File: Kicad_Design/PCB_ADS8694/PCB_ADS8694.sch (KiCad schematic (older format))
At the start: 46 parts, among them J1 Screw_Terminal_01x03_Alimenta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, J4 Conn_02x06_Male_Pmod_Spartan6, J5 Screw_Terminal_01x02_CH3, J6 Screw_Terminal_01x02_CH2, J7 Screw_Terminal_01x02_CH1, J8 Screw_Terminal_01x02_CH0, U1 LM7805_TO220, U2 AD8221, U3 AD8221, U4 ADS8694, U5 AD8221, U6 AD8221

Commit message: PCB V1
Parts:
- removed U4: ADS8694, Package_SO:TSSOP-38_4.4x9.7mm_P0.5mm, symbol PCB_ADS8694-rescue:ADS8694-Analog_ADC-PCB_ADS8694-rescue
- added U4: ADS8694_Vers2, Package_SO:TSSOP-38_4.4x9.7mm_P0.5mm, symbol ads8694_vers2:ADS8694_Vers2
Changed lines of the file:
@@
 EESchema Schematic File Version 4
-LIBS:PCB_ADS8694-cache
 EELAYER 29 0
 EELAYER END
@@
 F 3 "~" H 4950 1850 50  0001 C CNN
 	1    4950 1850
-	1    0    0    -1
-$EndComp
-$Comp
-L PCB_ADS8694-rescue:ADS8694-Analog_ADC-PCB_ADS8694-rescue U4
-U 1 1 5CCB2EF2
-P 5750 4500
-F 0 "U4" H 5750 4550 50  0000 C CNN
-F 1 "ADS8694" H 5750 4450 50  0000 C CNN
-F 2 "Package_SO:TSSOP-38_4.4x9.7mm_P0.5mm" H 5750 4500 50  0001 C CNN
-F 3 "http://www.ti.com/lit/ds/symlink/ads8694.pdf" H 6700 5800 50  0001 C CNN
-	1    5750 4500
 	1    0    0    -1
 $EndComp
@@
 L power:GNDD #PWR0119
 U 1 1 5CD863F9
-P 6100 5800
-F 0 "#PWR0119" H 6100 5550 50  0001 C CNN
-F 1 "GNDD" H 6104 5645 50  0000 C CNN
-F 2 "" H 6100 5800 50  0001 C CNN
-F 3 "" H 6100 5800 50  0001 C CNN
-	1    6100 5800
+P 6050 5800
+F 0 "#PWR0119" H 6050 5550 50  0001 C CNN
+F 1 "GNDD" H 6054 5645 50  0000 C CNN
+F 2 "" H 6050 5800 50  0001 C CNN
+F 3 "" H 6050 5800 50  0001 C CNN
+	1    6050 5800
 	1    0    0    -1
 $EndComp
@@
 Text GLabel 5750 3100 1    50   Input ~ 0
 AVDD
-Wire Wire Line
-	5650 5800 5650 5875
-Wire Wire Line
-	5450 5875 5450 5800
-Wire Wire Line
-	5550 5800 5550 5875
-Connection ~ 5550 5875
-Wire Wire Line
-	5550 5875 5450 5875
 $Comp
 L power:GNDA #PWR034
 U 1 1 5CEF30B1
-P 5650 5875
-F 0 "#PWR034" H 5650 5625 50  0001 C CNN
-F 1 "GNDA" H 5655 5702 50  0000 C CNN
-F 2 "" H 5650 5875 50  0001 C CNN
-F 3 "" H 5650 5875 50  0001 C CNN
-	1    5650 5875
-	1    0    0    -1
-$EndComp
-Wire Wire Line
-	5750 5800 5750 5875
-Wire Wire Line
-	5750 5875 5650 5875
-Connection ~ 5650 5875
-Wire Wire Line
-	5850 5800 5850 5875
-Wire Wire Line
-	5850 5875 5750 5875
-Connection ~ 5750 5875
-Wire Wire Line
-	5550 5875 5650 5875
+P 5600 5900
+F 0 "#PWR034" H 5600 5650 50  0001 C CNN
+F 1 "GNDA" H 5605 5727 50  0000 C CNN
+F 2 "" H 5600 5900 50  0001 C CNN
+F 3 "" H 5600 5900 50  0001 C CNN
+	1    5600 5900
+	1    0    0    -1
+$EndComp
 $Comp
 L Device:C C7
@@
 Text GLabel 4750 1750 0    50   Input ~ 0
 CS
+$Comp
+L ads8694_vers2:ADS8694_Vers2 U4
+U 1 1 5CE32CBF
+P 5750 4500
+F 0 "U4" H 5750 5981 50  0000 C CNN
+F 1 "ADS8694_Vers2" H 5750 5890 50  0000 C CNN
+F 2 "Package_SO:TSSOP-38_4.4x9.7mm_P0.5mm" H 5750 4500 50  0001 C CNN
+F 3 "http://www.ti.com/lit/ds/symlink/ads8694.pdf" H 6700 5800 50  0001 C CNN
+	1    5750 4500
+	1    0    0    -1
+$EndComp
+Wire Wire Line
+	5400 5800 5400 5900
+Wire Wire Line
+	5400 5900 5500 5900
+Wire Wire Line
+	5500 5800 5500 5900
+Connection ~ 5500 5900
+Wire Wire Line
+	5500 5900 5600 5900
+Wire Wire Line
+	5600 5800 5600 5900
+Connection ~ 5600 5900
+Wire Wire Line
+	5700 5800 5700 5900
+Wire Wire Line
+	5700 5900 5625 5900
+Wire Wire Line
+	5800 5800 5800 5900
+Wire Wire Line
+	5800 5900 5700 5900
+Connection ~ 5700 5900
 $EndSCHEMATC

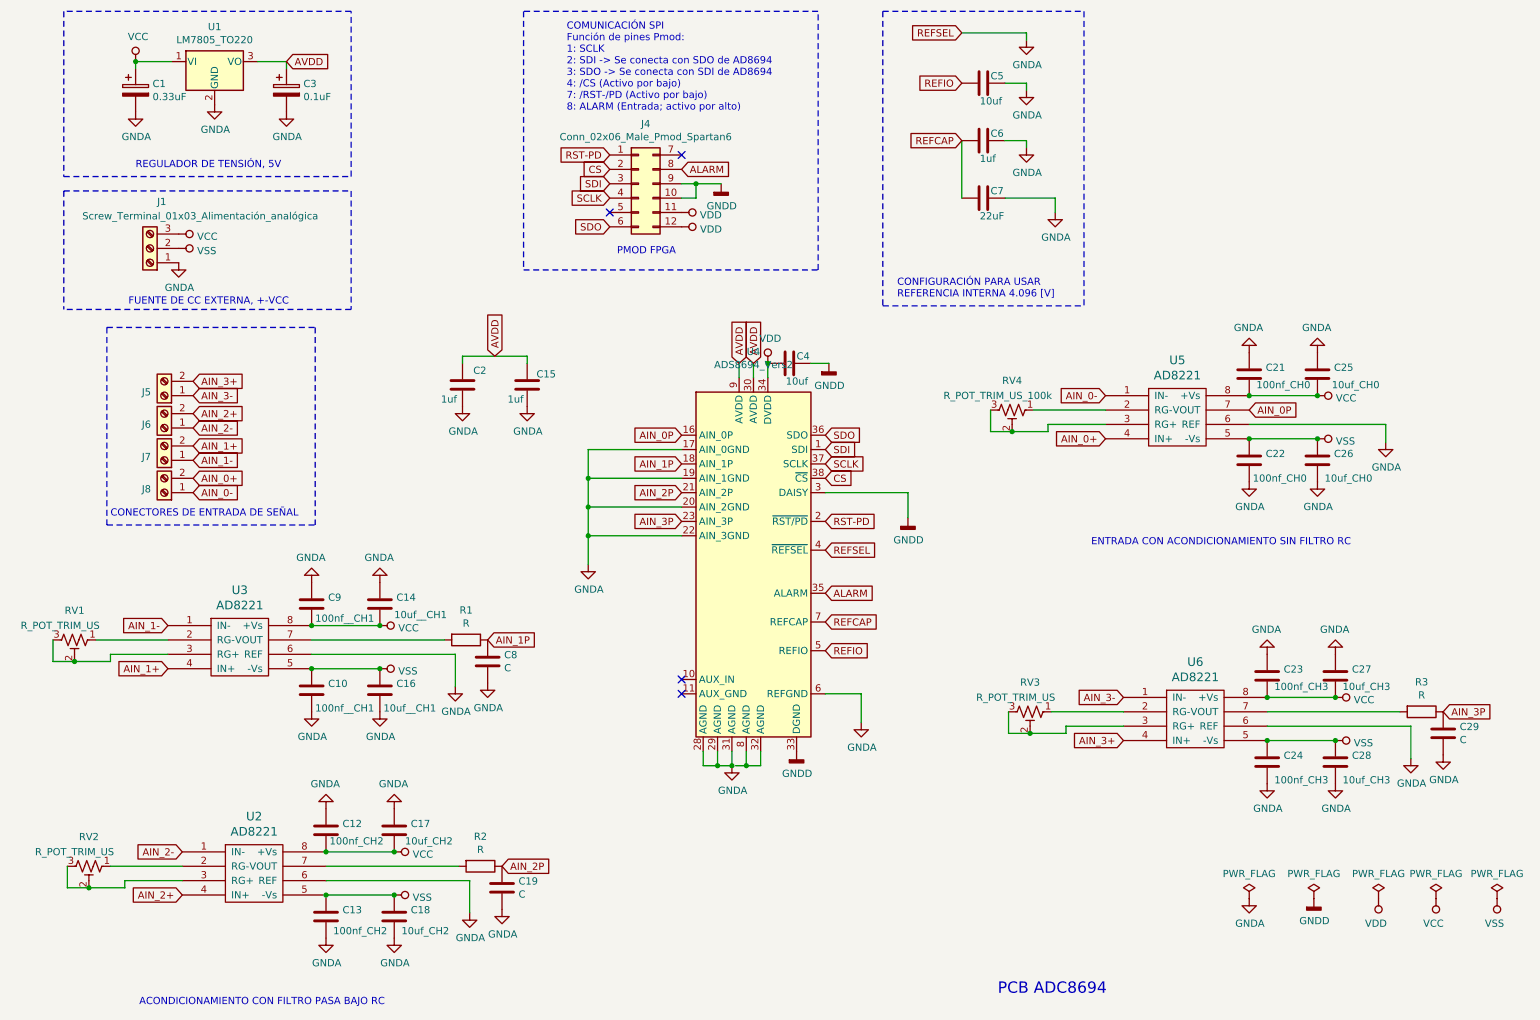
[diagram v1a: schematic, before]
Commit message: PCB V1
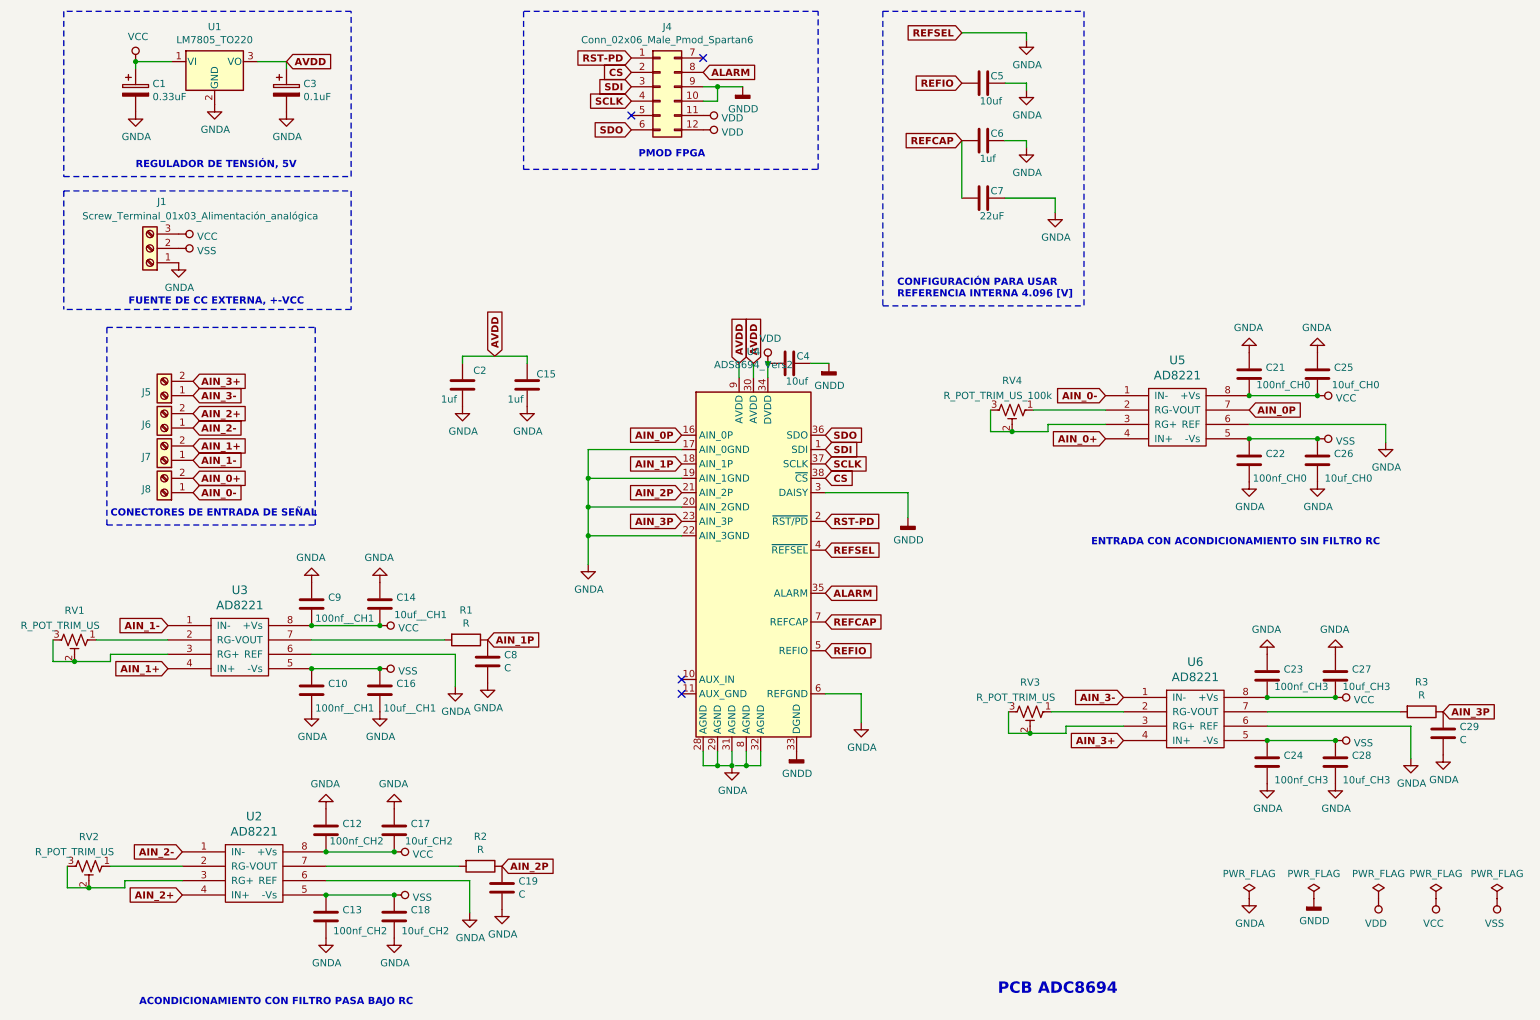
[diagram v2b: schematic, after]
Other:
- note removed: "COMUNICACIÓN SPI\nFunción de pines Pmod:\n1: SCLK\n2: SDI -> Se conecta con SDO de AD8694\n3: SDO -> Se conecta con SDI de AD8694\n4: /CS (Activo por bajo)\n7: /RST-/PD (Activo por bajo)\n8: ALARM (Entrada; activo por alto)"
- moved on the sheet: J4
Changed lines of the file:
@@
 L Connector_Generic:Conn_02x06_Top_Bottom J4
 U 1 1 5CCB59D8
-P 4950 1850
-F 0 "J4" H 5000 2267 50  0000 C CNN
-F 1 "Conn_02x06_Male_Pmod_Spartan6" H 5000 2176 50  0000 C CNN
-F 2 "Connector_PinHeader_2.54mm:PinHeader_2x06_P2.54mm_Horizontal" H 4950 1850 50  0001 C CNN
-F 3 "~" H 4950 1850 50  0001 C CNN
-	1    4950 1850
+P 5100 1175
+F 0 "J4" H 5150 1592 50  0000 C CNN
+F 1 "Conn_02x06_Male_Pmod_Spartan6" H 5150 1501 50  0000 C CNN
+F 2 "Connector_PinHeader_2.54mm:PinHeader_2x06_P2.54mm_Horizontal" H 5100 1175 50  0001 C CNN
+F 3 "~" H 5100 1175 50  0001 C CNN
+	1    5100 1175
 	1    0    0    -1
 $EndComp
@@
 Wire Wire Line
 	2500 1000 2500 1050
-Text GLabel 6250 4400 2    50   Input ~ 0
+Text GLabel 6250 4400 2    50   Input ~ 6
 REFSEL
-Text GLabel 6250 4700 2    50   Input ~ 0
+Text GLabel 6250 4700 2    50   Input ~ 6
 ALARM
-Text GLabel 6250 4900 2    50   Input ~ 0
+Text GLabel 6250 4900 2    50   Input ~ 6
 REFCAP
-Text GLabel 6250 5100 2    50   Input ~ 0
+Text GLabel 6250 5100 2    50   Input ~ 6
 REFIO
-Text GLabel 6250 4200 2    50   Input ~ 0
+Text GLabel 6250 4200 2    50   Input ~ 6
 RST-PD
-Text GLabel 6250 3900 2    50   Input ~ 0
+Text GLabel 6250 3900 2    50   Input ~ 6
 CS
-Text GLabel 6250 3800 2    50   Input ~ 0
+Text GLabel 6250 3800 2    50   Input ~ 6
 SCLK
-Text GLabel 6250 3700 2    50   Input ~ 0
+Text GLabel 6250 3700 2    50   Input ~ 6
 SDI
-Text GLabel 6250 3600 2    50   Input ~ 0
+Text GLabel 6250 3600 2    50   Input ~ 6
 SDO
-Text GLabel 5250 3800 0    50   Input ~ 0
+Text GLabel 5250 3800 0    50   Input ~ 6
 AIN_1P
-Text GLabel 5250 4000 0    50   Input ~ 0
+Text GLabel 5250 4000 0    50   Input ~ 6
 AIN_2P
-Text GLabel 5250 4200 0    50   Input ~ 0
+Text GLabel 5250 4200 0    50   Input ~ 6
 AIN_3P
-Text GLabel 7200 800  0    50   Input ~ 0
+Text GLabel 7200 800  0    50   Input ~ 6
 REFSEL
-Text GLabel 7200 1150 0    50   Input ~ 0
+Text GLabel 7200 1150 0    50   Input ~ 6
 REFIO
-Text GLabel 7200 1550 0    50   Input ~ 0
+Text GLabel 7200 1550 0    50   Input ~ 6
 REFCAP
 Wire Wire Line
 	7200 1550 7200 1950
-Text Notes 6750 2650 0    50   ~ 0
+Text Notes 6750 2650 0    50   ~ 6
 CONFIGURACIÓN PARA USAR\nREFERENCIA INTERNA 4.096 [V]\n
-Text Notes 4800 2350 0    50   ~ 0
+Text Notes 4950 1675 0    50   ~ 6
 PMOD FPGA
 Wire Notes Line
@@
 Wire Notes Line
 	2950 650  950  650
-Text Notes 1450 1750 0    50   ~ 0
+Text Notes 1450 1750 0    50   ~ 6
 REGULADOR DE TENSIÓN, 5V\n
-Text Notes 7450 7500 0    79   ~ 0
+Text Notes 7450 7500 0    79   ~ 6
 PCB ADC8694
 Wire Notes Line
 	950  650  950  1800
-Text GLabel 4750 1950 0    50   Input ~ 0
+Text GLabel 4900 1275 0    50   Input ~ 6
 SCLK
-Text GLabel 4750 2150 0    50   Input ~ 0
+Text GLabel 4900 1475 0    50   Input ~ 6
 SDO
-Text GLabel 4750 1850 0    50   Input ~ 0
+Text GLabel 4900 1175 0    50   Input ~ 6
 SDI
-Text Notes 4450 1350 0    50   ~ 0
-COMUNICACIÓN SPI\nFunción de pines Pmod:\n1: SCLK\n2: SDI -> Se conecta con SDO de AD8694\n3: SDO -> Se conecta con SDI de AD8694\n4: /CS (Activo por bajo)\n7: /RST-/PD (Activo por bajo)\n8: ALARM (Entrada; activo por alto)
-Wire Notes Line
-	4150 2450 6200 2450
-Wire Notes Line
-	6200 2450 6200 650
 Wire Notes Line
 	6200 650  4150 650
-Text Notes 1400 2700 0    50   ~ 0
+Text Notes 1400 2700 0    50   ~ 6
 FUENTE DE CC EXTERNA, +-VCC
 Wire Notes Line
@@
 Wire Wire Line
 	5250 3700 4600 3700
-NoConn ~ 4750 2050
-NoConn ~ 5250 1650
+NoConn ~ 4900 1375
+NoConn ~ 5400 975
 $Comp
 L power:GNDD #PWR0118
 U 1 1 5CD843B0
-P 5525 1850
-F 0 "#PWR0118" H 5525 1600 50  0001 C CNN
-F 1 "GNDD" H 5529 1695 50  0000 C CNN
-F 2 "" H 5525 1850 50  0001 C CNN
-F 3 "" H 5525 1850 50  0001 C CNN
-	1    5525 1850
+P 5675 1175
+F 0 "#PWR0118" H 5675 925 50  0001 C CNN
+F 1 "GNDD" H 5679 1020 50  0000 C CNN
+F 2 "" H 5675 1175 50  0001 C CNN
+F 3 "" H 5675 1175 50  0001 C CNN
+	1    5675 1175
 	1    0    0    -1
 $EndComp
@@
 	1    0    0    -1
 $EndComp
-Text GLabel 9200 3425 2    50   Input ~ 0
+Text GLabel 9200 3425 2    50   Input ~ 6
 AIN_0P
-Text GLabel 8200 3625 0    50   Input ~ 0
+Text GLabel 8200 3625 0    50   Input ~ 6
 AIN_0+
-Text GLabel 8200 3325 0    50   Input ~ 0
+Text GLabel 8200 3325 0    50   Input ~ 6
 AIN_0-
 $Comp
@@
 	0    1    1    0
 $EndComp
-Text GLabel 8325 5425 0    50   Input ~ 0
+Text GLabel 8325 5425 0    50   Input ~ 6
 AIN_3-
-Text GLabel 8325 5725 0    50   Input ~ 0
+Text GLabel 8325 5725 0    50   Input ~ 6
 AIN_3+
 Connection ~ 1125 6750
@@
 	0    1    1    0
 $EndComp
-Text GLabel 1775 6500 0    50   Input ~ 0
+Text GLabel 1775 6500 0    50   Input ~ 6
 AIN_2-
-Text GLabel 1775 6800 0    50   Input ~ 0
+Text GLabel 1775 6800 0    50   Input ~ 6
 AIN_2+
 Connection ~ 1025 5175
@@
 	0    1    1    0
 $EndComp
-Text GLabel 1675 4925 0    50   Input ~ 0
+Text GLabel 1675 4925 0    50   Input ~ 6
 AIN_1-
-Text GLabel 1675 5225 0    50   Input ~ 0
+Text GLabel 1675 5225 0    50   Input ~ 6
 AIN_1+
 $Comp
@@
 	1    0    0    -1
 $EndComp
-Text Notes 8100 4375 0    50   ~ 0
+Text Notes 8100 4375 0    50   ~ 6
 ENTRADA CON ACONDICIONAMIENTO SIN FILTRO RC\n
-Text Notes 1275 4175 0    50   ~ 0
+Text Notes 1275 4175 0    50   ~ 6
 CONECTORES DE ENTRADA DE SEÑAL
 $Comp
 L power:VDD #PWR0112
 U 1 1 5CD79A34
-P 5250 2050
-F 0 "#PWR0112" H 5250 1900 50  0001 C CNN
-F 1 "VDD" V 5268 2177 50  0000 L CNN
-F 2 "" H 5250 2050 50  0001 C CNN
-F 3 "" H 5250 2050 50  0001 C CNN
-	1    5250 2050
+P 5400 1375
+F 0 "#PWR0112" H 5400 1225 50  0001 C CNN
+F 1 "VDD" V 5418 1502 50  0000 L CNN
+F 2 "" H 5400 1375 50  0001 C CNN
+F 3 "" H 5400 1375 50  0001 C CNN
+	1    5400 1375
 	0    1    1    0
 $EndComp
@@
 L power:VDD #PWR0116
 U 1 1 5CD7F938
-P 5250 2150
-F 0 "#PWR0116" H 5250 2000 50  0001 C CNN
-F 1 "VDD" V 5267 2278 50  0000 L CNN
-F 2 "" H 5250 2150 50  0001 C CNN
-F 3 "" H 5250 2150 50  0001 C CNN
-	1    5250 2150
+P 5400 1475
+F 0 "#PWR0116" H 5400 1325 50  0001 C CNN
+F 1 "VDD" V 5417 1603 50  0000 L CNN
+F 2 "" H 5400 1475 50  0001 C CNN
+F 3 "" H 5400 1475 50  0001 C CNN
+	1    5400 1475
 	0    1    1    0
 $EndComp
@@
 	1    0    0    -1
 $EndComp
-Text GLabel 2500 1000 2    50   Input ~ 0
+Text GLabel 2500 1000 2    50   Input ~ 6
 AVDD
-Text GLabel 5650 3100 1    50   Input ~ 0
+Text GLabel 5650 3100 1    50   Input ~ 6
 AVDD
 $Comp
@@
 Wire Wire Line
 	4600 3700 4600 3900
-Text GLabel 5250 3600 0    50   Input ~ 0
+Text GLabel 5250 3600 0    50   Input ~ 6
 AIN_0P
 $Comp
@@
 	0    1    1    0
 $EndComp
-Text GLabel 3900 5025 2    50   Input ~ 0
+Text GLabel 3900 5025 2    50   Input ~ 6
 AIN_1P
 $Comp
@@
 	0    1    1    0
 $EndComp
-Text GLabel 4000 6600 2    50   Input ~ 0
+Text GLabel 4000 6600 2    50   Input ~ 6
 AIN_2P
 $Comp
@@
 	0    1    1    0
 $EndComp
-Text GLabel 10550 5525 2    50   Input ~ 0
+Text GLabel 10550 5525 2    50   Input ~ 6
 AIN_3P
 $Comp
@@
 	1    0    0    -1
 $EndComp
-Text GLabel 5750 3100 1    50   Input ~ 0
+Text GLabel 5750 3100 1    50   Input ~ 6
 AVDD
 $Comp
@@
 	-1   0    0    1
 $EndComp
-Text GLabel 3950 3050 1    50   Input ~ 0
+Text GLabel 3950 3050 1    50   Input ~ 6
 AVDD
 Wire Wire Line
@@
 Wire Notes Line
 	1250 2850 1250 4225
-Text GLabel 1850 3225 2    50   Input ~ 0
+Text GLabel 1850 3225 2    50   Input ~ 6
 AIN_3+
-Text GLabel 1850 3325 2    50   Input ~ 0
+Text GLabel 1850 3325 2    50   Input ~ 6
 AIN_3-
-Text GLabel 1850 3450 2    50   Input ~ 0
+Text GLabel 1850 3450 2    50   Input ~ 6
 AIN_2+
-Text GLabel 1850 3550 2    50   Input ~ 0
+Text GLabel 1850 3550 2    50   Input ~ 6
 AIN_2-
-Text GLabel 1850 3675 2    50   Input ~ 0
+Text GLabel 1850 3675 2    50   Input ~ 6
 AIN_1+
-Text GLabel 1850 3775 2    50   Input ~ 0
+Text GLabel 1850 3775 2    50   Input ~ 6
 AIN_1-
-Text GLabel 1850 3900 2    50   Input ~ 0
+Text GLabel 1850 3900 2    50   Input ~ 6
 AIN_0+
-Text GLabel 1850 4000 2    50   Input ~ 0
+Text GLabel 1850 4000 2    50   Input ~ 6
 AIN_0-
-Text Notes 1475 7575 0    50   ~ 0
+Text Notes 1475 7575 0    50   ~ 6
 ACONDICIONAMIENTO CON FILTRO PASA BAJO RC
 Wire Notes Line
@@
 NoConn ~ 5250 5300
 Wire Wire Line
-	5250 1850 5350 1850
-Wire Wire Line
-	5250 1950 5350 1950
-Wire Wire Line
-	5350 1950 5350 1850
-Connection ~ 5350 1850
-Wire Wire Line
-	5350 1850 5525 1850
-Wire Notes Line
-	4150 650  4150 2450
+	5400 1175 5500 1175
+Wire Wire Line
+	5400 1275 5500 1275
+Wire Wire Line
+	5500 1275 5500 1175
+Connection ~ 5500 1175
+Wire Wire Line
+	5500 1175 5675 1175
 $Comp
 L power:GNDD #PWR0106
@@
 Wire Wire Line
 	6825 4000 6250 4000
-Text GLabel 4750 1650 0    50   Input ~ 0
+Text GLabel 4900 975  0    50   Input ~ 6
 RST-PD
-Text GLabel 5250 1750 2    50   Input ~ 0
+Text GLabel 5400 1075 2    50   Input ~ 6
 ALARM
-Text GLabel 4750 1750 0    50   Input ~ 0
+Text GLabel 4900 1075 0    50   Input ~ 6
 CS
 $Comp
@@
 	5800 5900 5700 5900
 Connection ~ 5700 5900
+Wire Notes Line
+	4150 650  4150 1750
+Wire Notes Line
+	4150 1750 6200 1750
+Wire Notes Line
+	6200 1750 6200 650
 $EndSCHEMATC
